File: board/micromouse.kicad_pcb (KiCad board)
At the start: 2 copper layers, 100 x 123 mm, 62 parts, among them J1 Power, J2 SERIAL, J3 PWR_SEL, J4 Front Sense, J5 Left Sense, J6 Right Sense, J7 Back Sense, M1 Left Motor, M2 Right Motor, SW1 SW_SPST, SW2 SW_Push, SW3 SW_DIP_x04, SW4 SW_Push, SW5 SW_Push, U1 ATmega328P-PU, U2 L7805, U3 drv8825, U4 drv8825, U5 CD4052B, Y1 16MHz

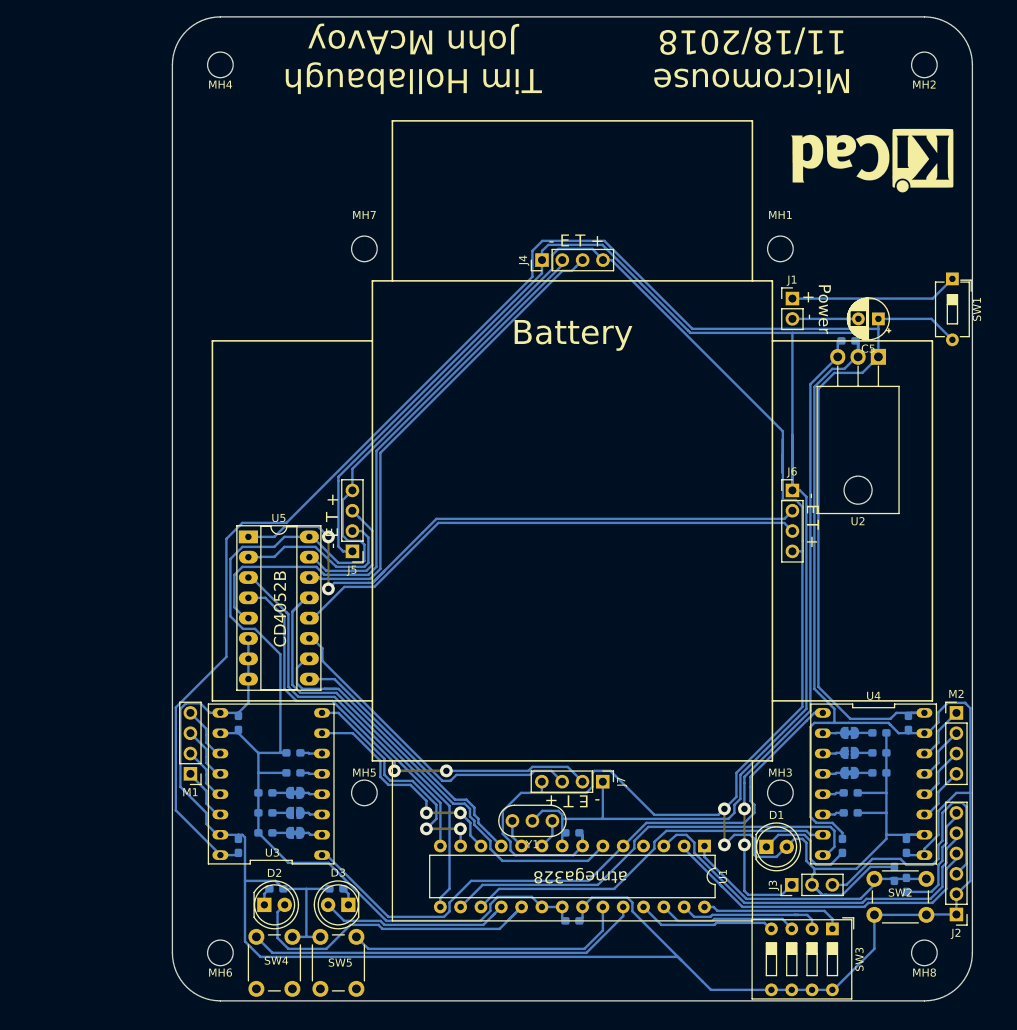
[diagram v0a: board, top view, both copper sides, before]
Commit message: Finished board layout
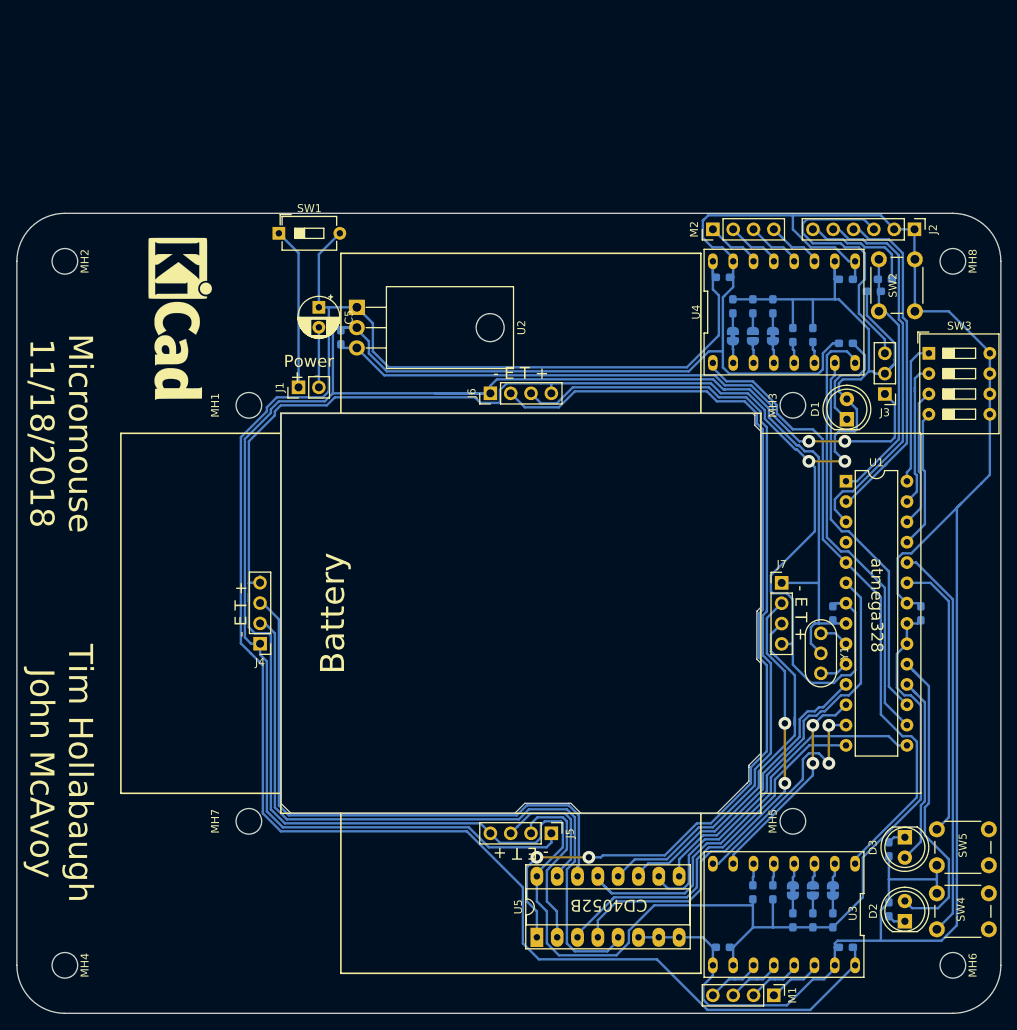
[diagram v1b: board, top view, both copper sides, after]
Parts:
- moved MH4 114.2 mm to (86.6, 155.6), turned to 90 degrees
- moved MH2 110.2 mm to (86.6, 67.6), turned to 90 degrees
- moved SW4 91.9 mm to (202.1, 151.1), turned to 180 degrees
- moved MH6 91.6 mm to (197.6, 155.6), turned to 90 degrees
- moved REF** 88.7 mm to (101.0, 74.8), turned to 270 degrees
- moved MH8 86.5 mm to (197.6, 67.6), turned to 90 degrees
- moved J2 85.8 mm to (192.8, 63.6), turned to 270 degrees
- moved SW1 84.4 mm to (113.3, 64.1), turned to 0 degrees
- moved D2 80.1 mm to (191.6, 150.1), turned to 90 degrees
- moved M1 78.0 mm to (175.2, 159.3), turned to 270 degrees
- moved C6 77.0 mm to (184.2, 153.3), turned to 180 degrees
- moved R13 76.6 mm to (189.6, 148.6), turned to 90 degrees
- moved C9 75.7 mm to (189.1, 69.8), turned to 0 degrees
- moved SW5 73.8 mm to (195.6, 138.6), turned to 0 degrees
- moved MH7 73.0 mm to (109.6, 137.6), turned to 90 degrees
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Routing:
- net /RIGHT_ECHO: track 81.7 -> 123.1 mm
- net /RIGHT_TRIG: track 65.7 -> 101.6 mm
- net +5V: track 398.7 -> 419.7 mm
- net +BATT: track 229.1 -> 244.7 mm
- net GND: track 537.4 -> 551.9 mm
- net /FRONT_TRIG: track 59.2 -> 73.2 mm
- net /FRONT_ECHO: track 73.7 -> 87.5 mm
- net /BACK_TRIG: track 41.0 -> 46.5 mm
- net /LEFT_STEP: track 28.7 -> 26.6 mm
- net /BACK_ECHO: track 57.6 -> 59.4 mm
- net /SENSE_SEL_1: track 33.5 -> 35.0 mm
- net /LEFT_DIR: track 30.2 -> 29.1 mm
- net Net-(J1-Pad1): track 21.0 -> 20.3 mm
- net Net-(C8-Pad1): track 81.4 -> 82.0 mm
- net /SENSE_TRIG: track 53.3 -> 53.9 mm
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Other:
- board size 100 x 123 mm -> 123 x 100 mm

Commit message: Finish small board
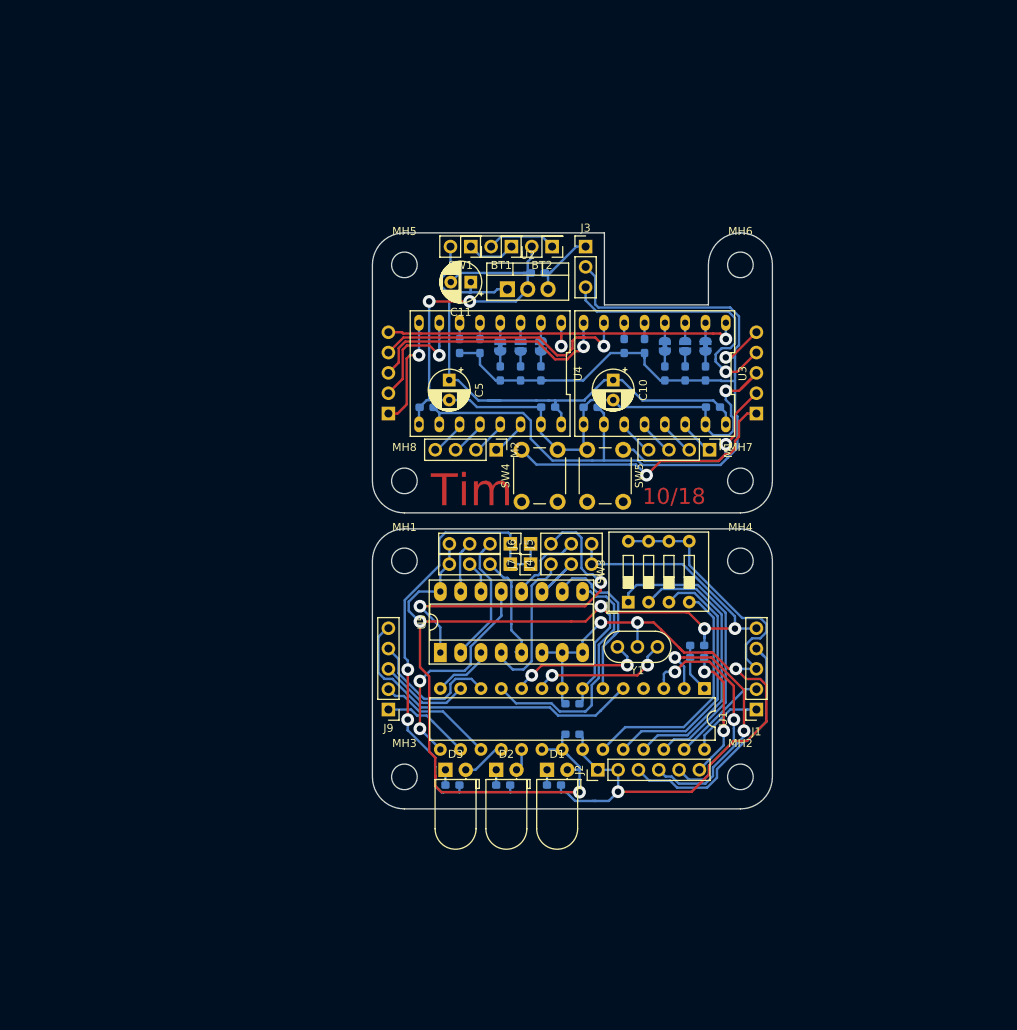
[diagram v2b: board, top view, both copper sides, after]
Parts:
- removed REF**: KiCad-Logo_8mm_SilkScreen, Symbol:KiCad-Logo_8mm_SilkScreen
- removed SW2: SW_Push, Button_Switch_THT:SW_PUSH_6mm
- removed svg2mod: G***, svg2mod:Rowan_Logo_Torch
- added BT1: 3x AA, Connector_PinHeader_2.54mm:PinHeader_2x01_P2.54mm_Vertical, F.Cu at (142.4, 65.7)
- added BT2: 3x AA, Connector_PinHeader_2.54mm:PinHeader_2x01_P2.54mm_Vertical, F.Cu at (147.5, 65.7)
- added C10: CP, Capacitor_THT:CP_Radial_D5.0mm_P2.50mm, F.Cu at (155.1, 82.4)
- added C11: CP, Capacitor_THT:CP_Radial_D5.0mm_P2.50mm, F.Cu at (137.3, 70.2)
- added J12: MotorsUpper, Connector_PinSocket_2.54mm:PinSocket_1x05_P2.54mm_Vertical, B.Cu at (127.0, 86.6)
- added J8: PowerBtnUpper, Connector_PinSocket_2.54mm:PinSocket_1x05_P2.54mm_Vertical, B.Cu at (173.0, 86.6)
- added J9: MotorsLower, Connector_PinHeader_2.54mm:PinHeader_1x05_P2.54mm_Vertical, F.Cu at (127.0, 123.6)
- D1, D2, D3: footprint LED_THT:LED_D5.0mm -> LED_THT:LED_D5.0mm_Horizontal_O1.27mm_Z3.0mm
- J1: value Power -> PowerBtnLower; footprint Connector_PinHeader_2.54mm:PinHeader_1x02_P2.54mm_Vertical -> Connector_PinSocket_2.54mm:PinSocket_1x05_P2.54mm_Vertical
- SW1: footprint Button_Switch_THT:SW_DIP_SPSTx01_Slide_6.7x4.1mm_W7.62mm_P2.54mm_LowProfile -> Connector_PinHeader_2.54mm:PinHeader_2x01_P2.54mm_Vertical
- U2: footprint Package_TO_SOT_THT:TO-220-3_Horizontal_TabDown -> Package_TO_SOT_THT:TO-220-3_Vertical
- moved MH2 106.2 mm to (171.0, 132.0), turned to 0 degrees
- moved MH4 98.4 mm to (171.0, 105.0), turned to 0 degrees
- moved MH6 91.5 mm to (171.0, 68.0), turned to 0 degrees
- moved MH5 84.8 mm to (129.0, 68.0), turned to 0 degrees
- moved SW4 79.2 mm to (143.7, 97.6), turned to 90 degrees
- moved J2 78.3 mm to (153.2, 131.1), turned to 90 degrees
- moved MH7 74.7 mm to (171.0, 95.0), turned to 0 degrees
- moved MH8 73.8 mm to (129.0, 95.0), turned to 0 degrees
- moved R4 70.2 mm to (161.6, 81.6)
- moved R3 70.2 mm to (164.1, 81.6)
- moved R2 70.2 mm to (166.6, 81.6)
- moved R6 70.2 mm to (156.5, 78.1)
- moved R5 70.1 mm to (159.0, 78.1)
- moved J1 70.0 mm to (173.0, 123.6), turned to 180 degrees
- moved JP3 69.9 mm to (161.6, 78.2)
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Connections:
- C1 pad 1: +5V -> +5VD
- C1 pad 2: GND -> GNDD
- C2 pad 1: +5V -> +5VD
- C2 pad 2: GND -> GNDD
- D1 pad 2: +5V -> +5VD
- J1 pad 1: Net-(J1-Pad1) -> /BTN1
- J1 pad 2: GND -> /BTN2
- J2 pad 1: GND -> GNDD
- J2 pad 2: GND -> GNDD
- J3 pad 3: /USB_5V -> /USB_5V_T
- J4 pad 1: GND -> GNDD
- J4 pad 4: +5V -> +5VD
- J5 pad 1: GND -> GNDD
- J5 pad 4: +5V -> +5VD
- J6 pad 1: GND -> GNDD
- J6 pad 4: +5V -> +5VD
- J7 pad 1: GND -> GNDD
- J7 pad 4: +5V -> +5VD
- R1 pad 2: +5V -> +5VD
- R12 pad 2: GND -> GNDD
- R13 pad 2: GND -> GNDD
- R14 pad 2: GND -> GNDD
- SW1 pad 1: Net-(J1-Pad1) -> Net-(BT1-Pad1)
- SW3 pad 5: GND -> GNDD
- SW3 pad 6: GND -> GNDD
- SW3 pad 7: GND -> GNDD
- SW3 pad 8: GND -> GNDD
- SW4 pad 1: /BTN1 -> /BTN1_T
- SW5 pad 1: /BTN2 -> /BTN2_T
- U1 pad 20: +5V -> +5VD
- U1 pad 21: +5V -> +5VD
- U1 pad 22: GND -> GNDD
- U1 pad 23: /BTN2 -> Net-(SW3-Pad4)
- U1 pad 24: /BTN1 -> Net-(SW3-Pad3)
- U1 pad 25: Net-(SW3-Pad4) -> Net-(SW3-Pad2)
- U1 pad 26: Net-(SW3-Pad3) -> Net-(SW3-Pad1)
- U1 pad 27: Net-(SW3-Pad2) -> /BTN2
- U1 pad 28: Net-(SW3-Pad1) -> /BTN1
- U1 pad 7: +5V -> +5VD
- U1 pad 8: GND -> GNDD
- U3 pad 1: /M_ENABLE -> /M_ENABLE_T
- U3 pad 7: /LEFT_STEP -> /LEFT_STEP_T
- U3 pad 8: /LEFT_DIR -> /LEFT_DIR_T
- U4 pad 1: /M_ENABLE -> /M_ENABLE_T
- U4 pad 7: /RIGHT_STEP -> /RIGHT_STEP_T
- U4 pad 8: /RIGHT_DIR -> /RIGHT_DIR_T
- U5 pad 16: +5V -> +5VD
- U5 pad 6: GND -> GNDD
- U5 pad 7: GND -> GNDD
- U5 pad 8: GND -> GNDD
- Y1 pad 2: GND -> GNDD
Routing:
- net GND: track 551.9 -> 110.7 mm, vias 0 -> 3
- net +5V: track 419.7 -> 140.1 mm, vias 2 -> 1
- net GNDD: track 0.00 -> 196.4 mm, vias 0 -> 6
- net +BATT: track 244.7 -> 73.2 mm
- net +5VD: track 0.00 -> 153.5 mm, vias 0 -> 5
- net /RIGHT_TRIG: track 101.6 -> 10.2 mm
- net /RIGHT_ECHO: track 123.1 -> 43.0 mm
- net /FRONT_ECHO: track 87.5 -> 14.2 mm
- net Net-(C8-Pad1): track 82.0 -> 8.96 mm, vias 2 -> 0
- net /FRONT_TRIG: track 73.2 -> 4.01 mm
- net /M_ENABLE_T: track 0.00 -> 49.1 mm, vias 0 -> 2
- net /RIGHT_DIR: track 55.5 -> 11.2 mm
- net /BACK_ECHO: track 59.4 -> 18.5 mm, vias 2 -> 0
- net /M_ENABLE: track 80.9 -> 40.4 mm
- net /SENSE_ECHO: track 47.3 -> 6.83 mm
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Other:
- board size 123 x 100 mm -> 50 x 72 mm
- board text added: "10/18"
- board text added: "Tim"
- board text removed: "+"
- board text removed: "-"
- board text removed: "- E T +"
- board text removed: "Battery"
- board text removed: "CD4052B"
- board text removed: "Micromouse 11/18/2018"
- board text removed: "Power"
- board text removed: "Tim Hollabaugh John McAvoy"
- board text removed: "atmega328"
